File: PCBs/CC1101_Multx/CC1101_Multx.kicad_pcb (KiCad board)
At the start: 4 copper layers, 34.7 x 26.8 mm, 49 parts, among them IC1 CC1101RGPR, IC2 ASWD-S2-0005-T, IC3 ASWD-S2-0005-T, IC4 ASWD-S2-0005-T, J1 MCU, J2 MCU, J3 MCU, J4 MCU, J5 MCU, J6 MCU, J7 MCU, J8 MCU, J9 MCU, Y1 XRCGB26M000F1S2BR0

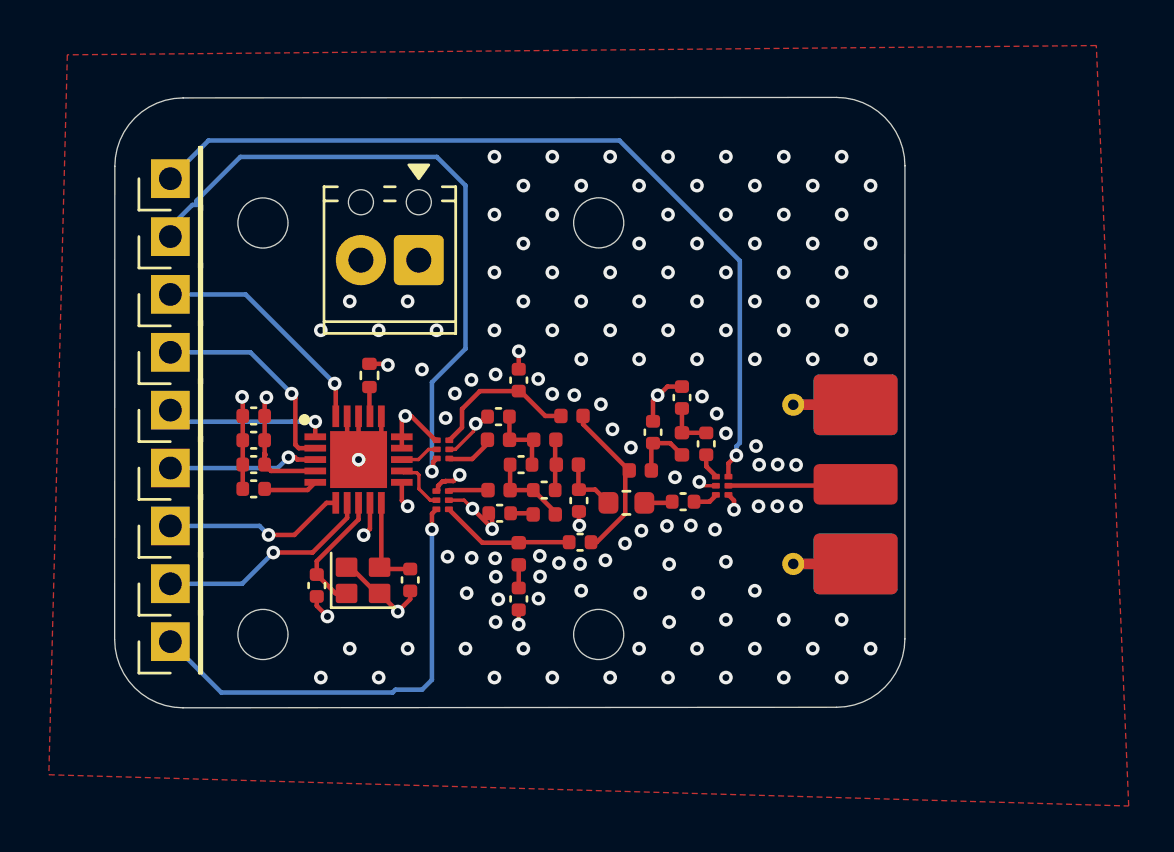
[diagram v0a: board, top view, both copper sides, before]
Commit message: V3 Fasivel
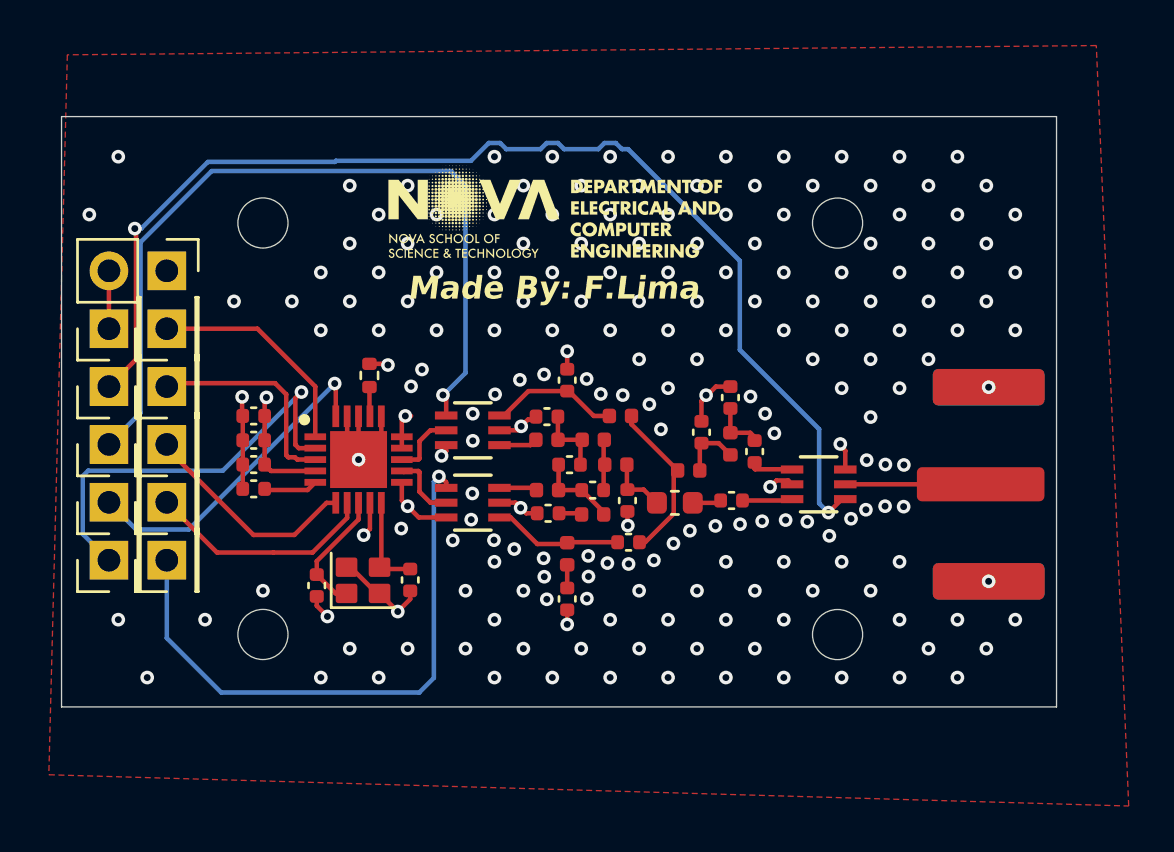
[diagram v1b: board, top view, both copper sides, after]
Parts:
- removed IC2, IC3, IC4: ASWD-S2-0005-T, Library:ASWS_S2_0002
- removed the REF** at (167.1, 89.5)
- removed the REF** at (167.1, 71.5)
- added J1: MCU, Connector_PinHeader_2.54mm:PinHeader_1x01_P2.54mm_Vertical, F.Cu at (145.6, 76.1)
- added REF**: MountingHole_2.2mm_M2_DIN965, MountingHole:MountingHole_2.2mm_M2_DIN965, F.Cu at (177.6, 71.5)
- added REF**: MountingHole_2.2mm_M2_DIN965, MountingHole:MountingHole_2.2mm_M2_DIN965, F.Cu at (177.6, 89.6)
- added U1: 4259-63, Library:SC-70-6_PSM-M, F.Cu at (161.6, 80.6)
- added U2: 4259-63, Library:SC-70-6_PSM-M, F.Cu at (176.8, 83.0)
- added U3: 4259-63, Library:SC-70-6_PSM-M, F.Cu at (161.6, 83.8)
- AE1: footprint Connector_Coaxial:SMA_Molex_73251-2120_EdgeMount_Horizontal -> Library:SMA_CONSMA020_062_G
- BT1: footprint TerminalBlock_Phoenix:TerminalBlock_Phoenix_MPT-0,5-2-2.54_1x02_P2.54mm_Horizontal -> Connector_PinHeader_2.54mm:PinHeader_1x02_P2.54mm_Vertical
- moved BT1 11.1 mm to (148.2, 73.6), turned to -90 degrees
- moved J2 9.51 mm to (145.6, 86.3)
- moved J9 9.51 mm to (145.6, 78.7)
- moved J4 9.51 mm to (145.6, 83.8)
- moved J7 9.51 mm to (145.6, 81.2)
- moved AE1 5.24 mm to (183.9, 83.0)
- moved J1 3.58 mm to (148.2, 76.1)
- moved J5 3.58 mm to (148.2, 81.2)
- moved J3 3.58 mm to (148.2, 78.7)
- moved J6 3.58 mm to (148.2, 83.8)
- moved J8 3.58 mm to (148.2, 86.3)
- moved C125_1 2.15 mm to (174.0, 81.5)
- moved C125_2 2.13 mm to (173.0, 83.7)
- moved C123_1 2.13 mm to (172.9, 79.2)
- moved C124_1 2.13 mm to (165.8, 88.0)
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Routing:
- net Net-(J9-Pin_1): track 37.5 -> 51.8 mm, vias 1 -> 2
- net Net-(IC1-SO_(GDO1)): track 9.32 -> 18.7 mm
- net Net-(J7-Pin_1): track 29.0 -> 35.8 mm
- net Net-(J8-Pin_1): track 20.2 -> 26.1 mm
- net Net-(IC1-SI): track 10.3 -> 14.5 mm
- net Net-(IC1-GDO2): track 6.60 -> 9.53 mm, vias 1 -> 0
- net Net-(IC1-SCLK): track 7.24 -> 9.77 mm, vias 1 -> 0
- net Net-(IC1-GDO0_(ATEST)): track 8.01 -> 9.74 mm, vias 1 -> 0
- net /RF_N: track 1.72 -> 3.14 mm
- net /868_A: track 1.07 -> 2.20 mm
- net /433_N: track 6.71 -> 5.72 mm
- net /433_A: track 1.11 -> 1.94 mm
- net /RF_P: track 2.40 -> 3.16 mm
- net /To_Ant: track 6.18 -> 6.91 mm
- net /AVDD: track 14.0 -> 13.4 mm
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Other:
- board size 34.7 x 26.8 mm -> 43.7 x 25.9 mm
- board text added: "Made By: F.Lima"

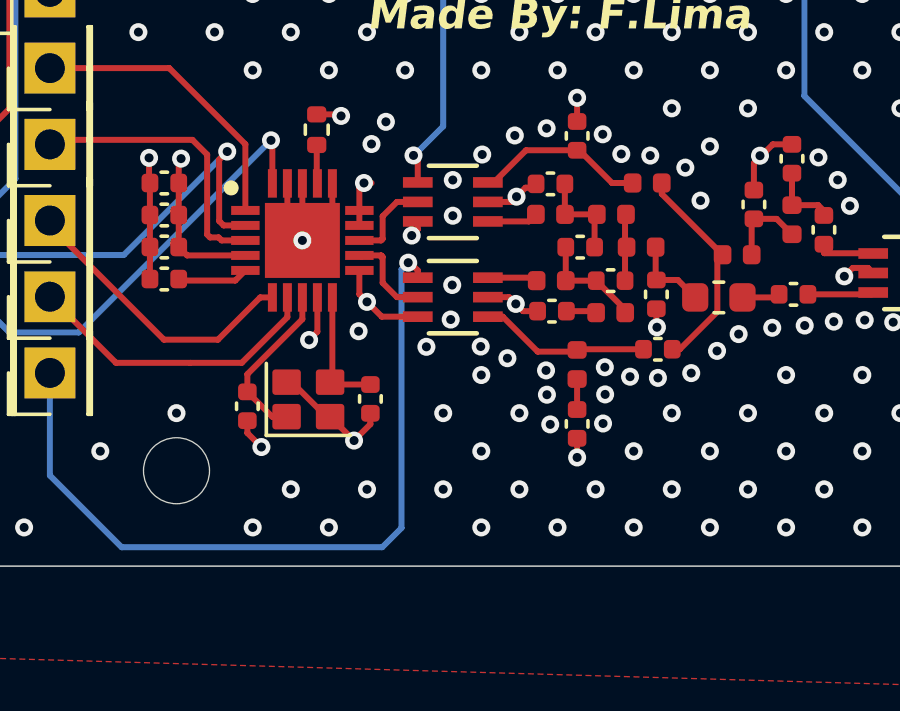
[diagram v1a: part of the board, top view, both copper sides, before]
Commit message: pord please
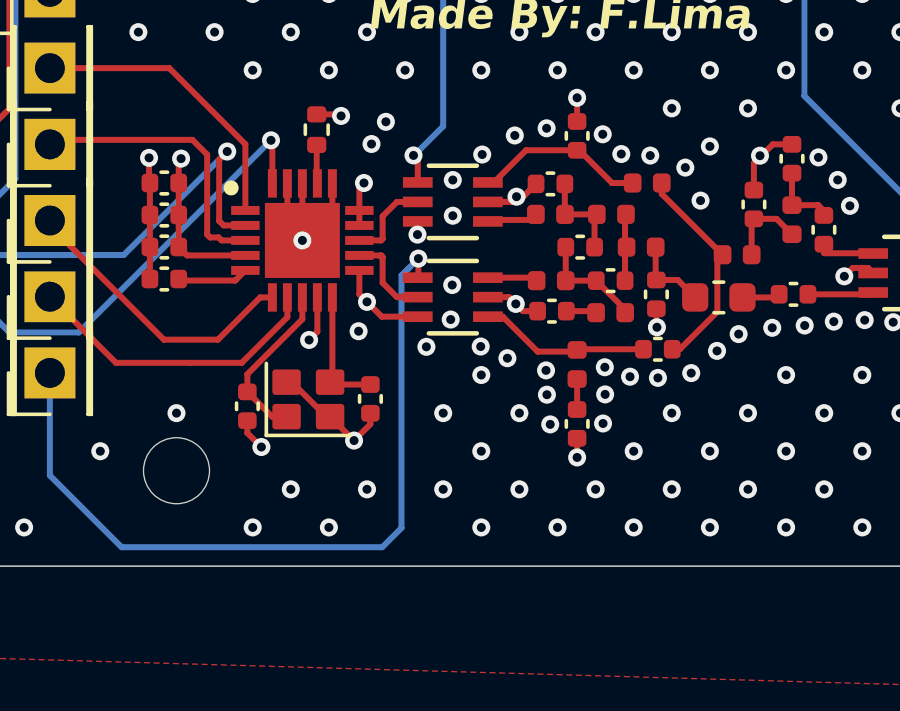
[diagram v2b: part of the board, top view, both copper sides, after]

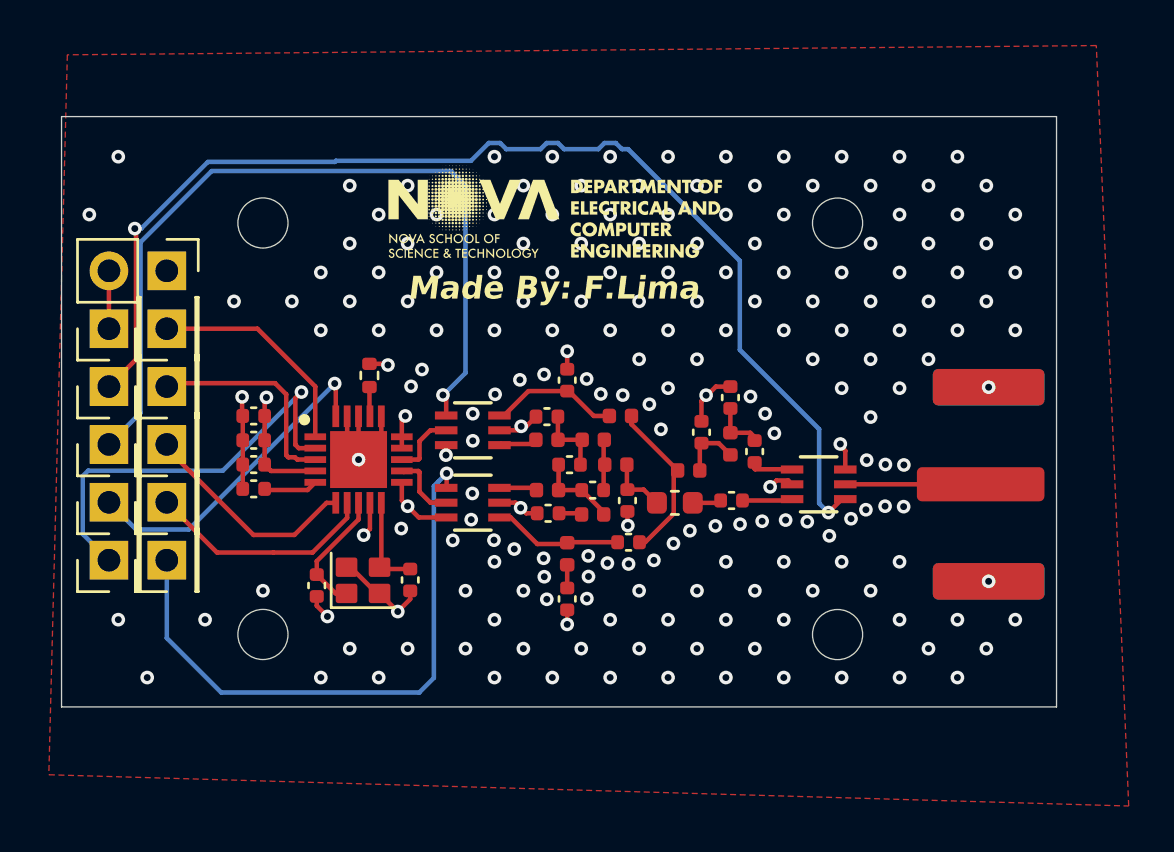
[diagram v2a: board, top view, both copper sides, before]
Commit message: 2ants prod
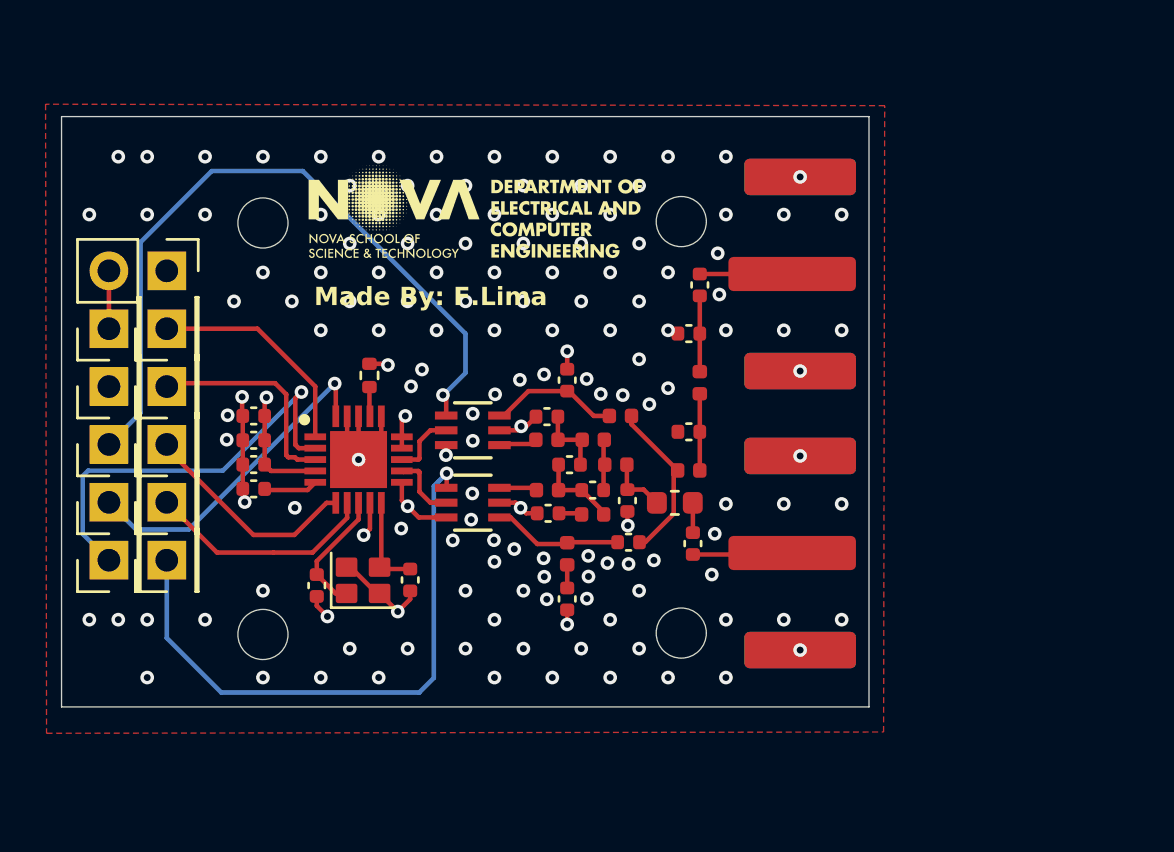
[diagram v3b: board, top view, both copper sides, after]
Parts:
- removed U2: 4259-63, Library:SC-70-6_PSM-M
- added AE2: Antenna_Shield, Library:SMA_CONSMA020_062_G, F.Cu at (175.6, 86.0)
- moved AE1 12.4 mm to (175.6, 73.7)
- moved C125_1 7.70 mm to (171.6, 74.2), turned to -90 degrees
- moved REF** 6.86 mm to (170.8, 71.4)
- moved REF** 6.86 mm to (170.8, 89.5)
- moved C123_1 3.35 mm to (171.1, 76.3), turned to 0 degrees
- moved L123_1 3.00 mm to (171.6, 78.5)
- moved C125_2 2.54 mm to (171.3, 85.6), turned to 90 degrees
- moved C122_1 0.55 mm to (171.1, 80.7), turned to 0 degrees
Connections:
- AE1 pad 1: /To_Ant -> /433_A
- J9 pad 1: Net-(J9-Pin_1) -> /AGND
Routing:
- net Net-(J9-Pin_1): track 51.8 -> 0.00 mm, vias 2 -> 0
- net /To_Ant: track 6.91 -> 0.00 mm
- net Net-(J7-Pin_1): track 35.8 -> 32.0 mm
- net /AGND: track 28.4 -> 24.8 mm, vias 195 -> 144
- net /868_A: track 2.20 -> 4.38 mm
- net /433_A: track 1.94 -> 4.05 mm
- net /AVDD: track 13.0 -> 11.8 mm, vias 6 -> 5
- net Net-(C123_1-Pad2): track 2.36 -> 3.33 mm
- net Net-(C122_1-Pad2): track 2.71 -> 3.37 mm
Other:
- board size 43.7 x 25.9 mm -> 35.4 x 25.9 mm
